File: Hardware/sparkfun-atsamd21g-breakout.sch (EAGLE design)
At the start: 41 parts, among them Q1 2N7002PW, Q3 2.5A/30V, U1 ATSAMD21G-A, U2 MIC5219 3.3V, U4 74AHC1G125

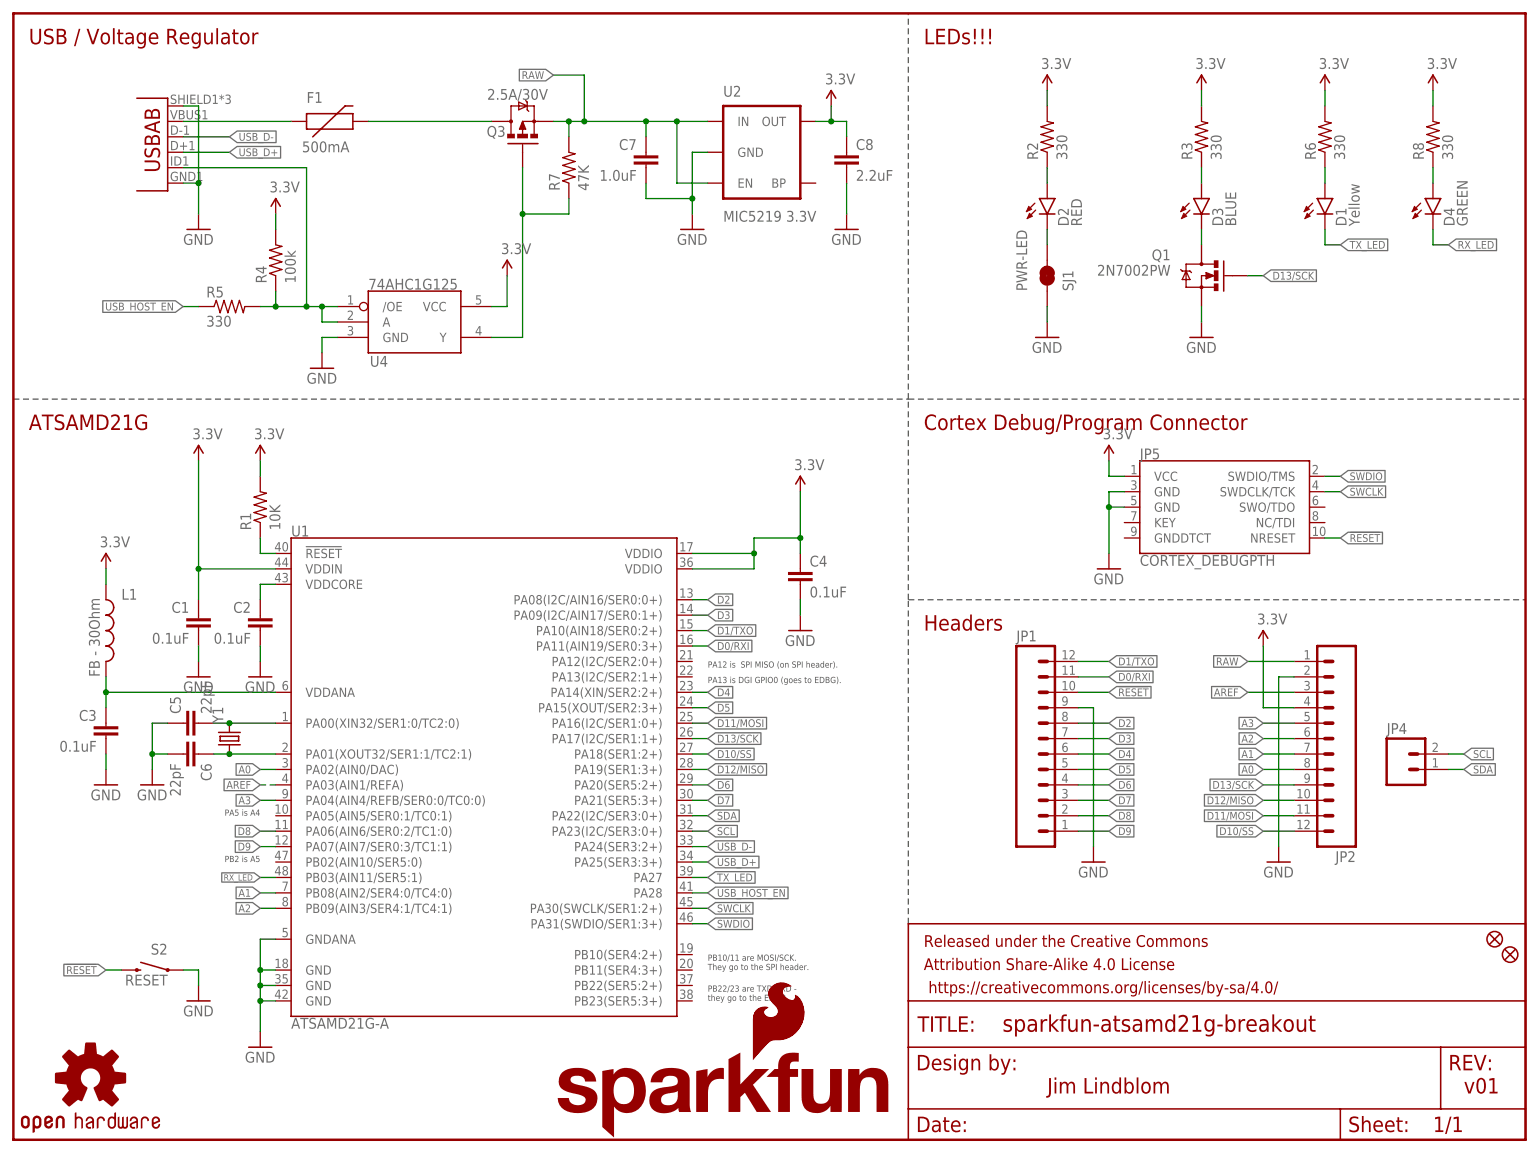
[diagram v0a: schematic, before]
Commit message: Minor, pre-checklist modifications.
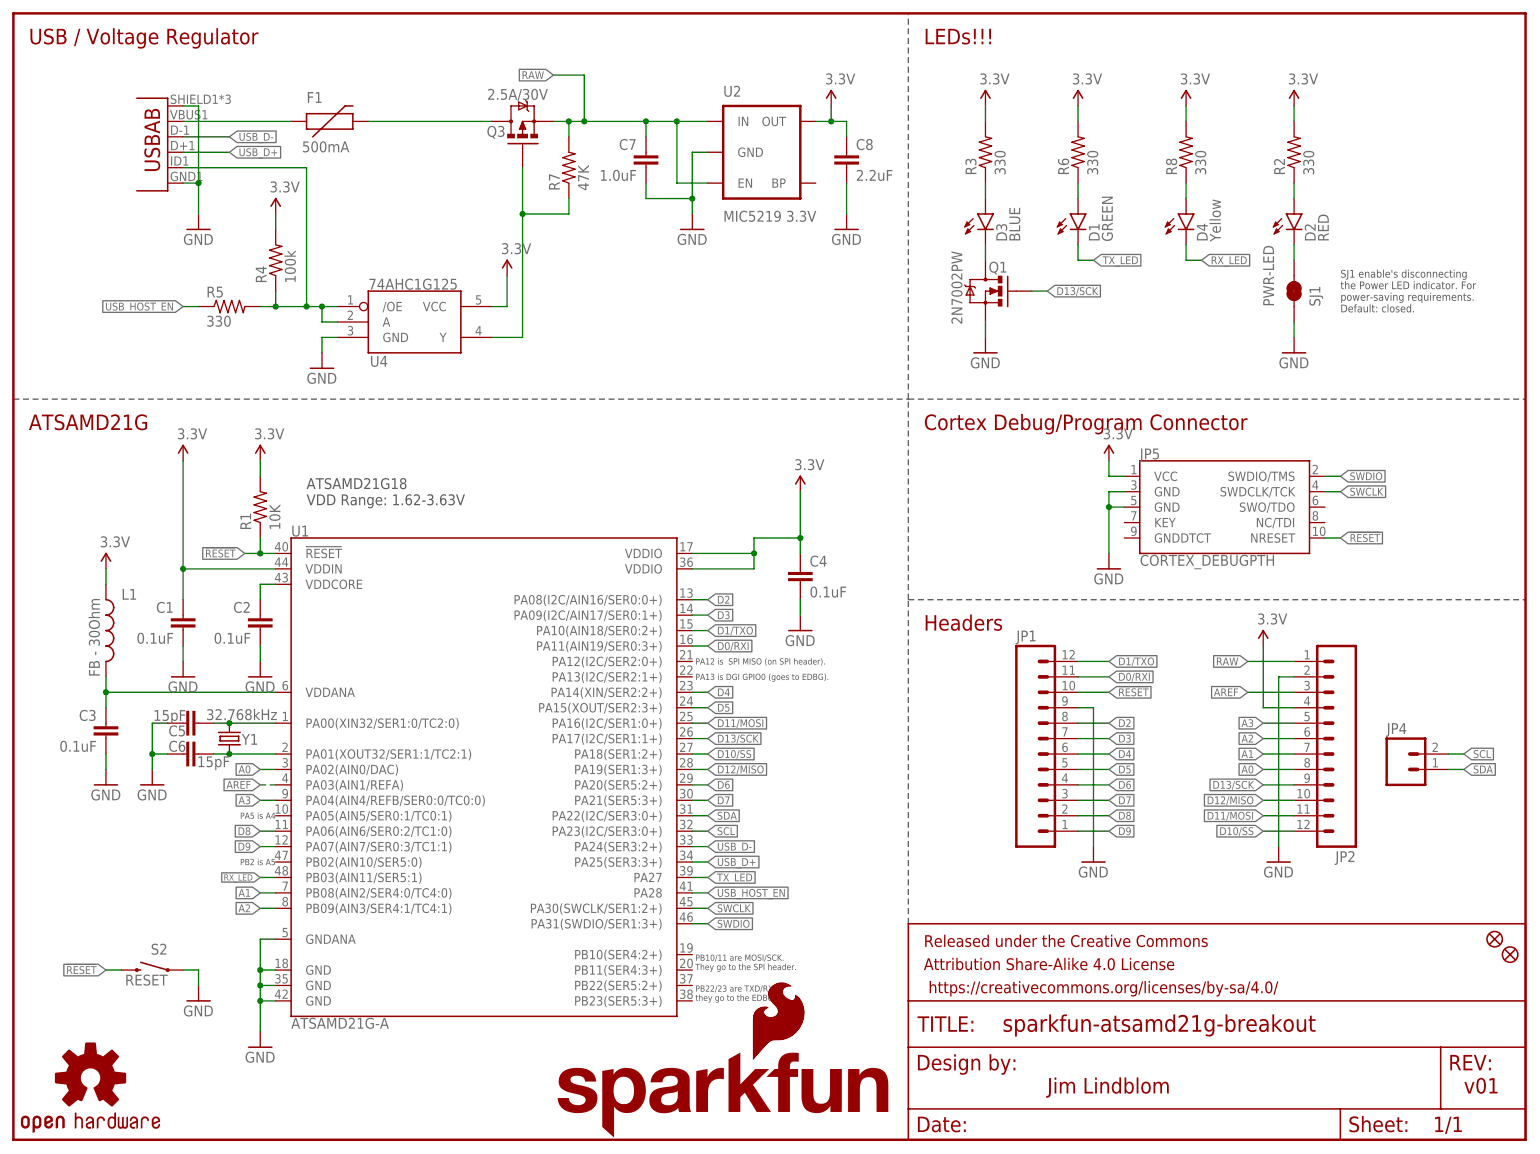
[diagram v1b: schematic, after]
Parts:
- C5, C6: value 22pF -> 15pF; device SparkFun-Capacitors:CAP0402-CAP -> samd21-temp:15PF-50V(+-5%)(0402)
- D1: value Yellow -> GREEN; device SparkFun-LED:LED-YELLOW0603 -> SparkFun-LED:LED-GREEN0603
- D4: value GREEN -> Yellow; device SparkFun-LED:LED-GREEN0603 -> SparkFun-LED:LED-YELLOW0603
- Y1: value (none) -> 32.768kHz
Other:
- note added: "ATSAMD21G18 VDD Range: 1.62-3.63V"
- note added: "SJ1 enable's disconnecting the Power LED indicator. For power-saving requirements. Default: closed."
- moved on the sheet: C1, D1, D2, D3, D4, Q1, R2, R3, R6, R8, SJ1
